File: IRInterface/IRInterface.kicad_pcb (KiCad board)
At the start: 2 copper layers, 27 x 33.5 mm, 25 parts, among them IC1 THVD1424RGTR, J2 RJHSE5E80, J3 FTSH-105-01-L-DV-007-K, Q1 SFH309, Q2 BC817, Q3 BC807, U1 74LVC1G17, U2 74LVC1G17, U3 STM32G030F6Px

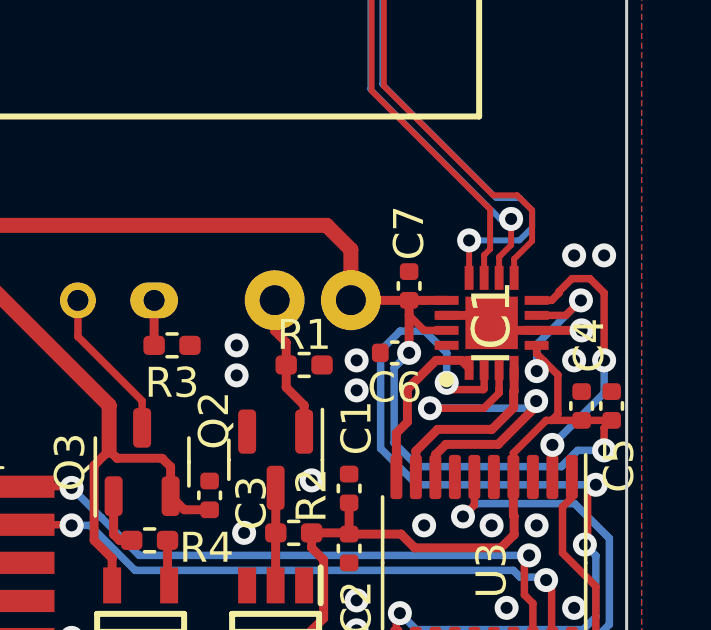
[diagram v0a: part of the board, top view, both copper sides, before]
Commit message: Fix review findings
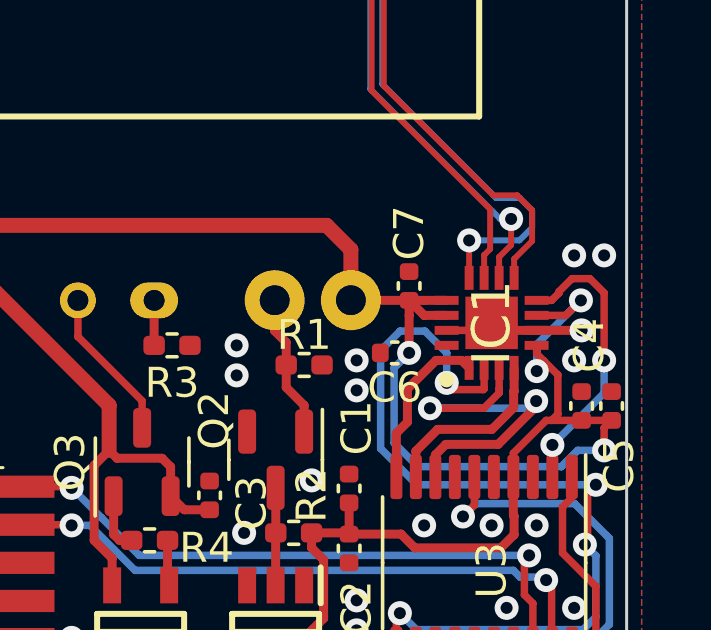
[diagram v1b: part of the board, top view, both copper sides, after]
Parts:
- R3: value 180R -> 150R
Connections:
- IC1 pad 14: GND -> VTref
- IC1 pad 15: VTref -> GND
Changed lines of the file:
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@@
         (effects (font (size 1 1) (thickness 0.15)))
     )
-    (fp_text value "180R" (at 0 1.17) (layer "F.Fab")
+    (fp_text value "150R" (at 0 1.17) (layer "F.Fab")
         (effects (font (size 1 1) (thickness 0.15)))
     )
@@
       (net 9 "DI+") (pinfunction "6") (pintype "passive"))
     (pad "7" thru_hole circle (at -6.09 0 180) (size 1.446 1.446) (drill 0.89) (layers "*.Cu" "*.Mask")
-      (net 15 "unconnected-(J2-Pad7)") (pinfunction "7") (pintype "passive"))
+      (net 15 "unconnected-(J2-Pad7)") (pinfunction "7") (pintype "passive+no_connect"))
     (pad "8" thru_hole circle (at -7.11 -1.78 180) (size 1.446 1.446) (drill 0.89) (layers "*.Cu" "*.Mask")
-      (net 16 "unconnected-(J2-Pad8)") (pinfunction "8") (pintype "passive"))
+      (net 16 "unconnected-(J2-Pad8)") (pinfunction "8") (pintype "passive+no_connect"))
     (pad "MH1" thru_hole circle (at 4.575 -0.89 180) (size 2.355 2.355) (drill 1.57) (layers "*.Cu" "*.Mask")
       (net 2 "GND") (pinfunction "MH1") (pintype "passive"))
@@
       (net 34 "VTref") (pinfunction "VIO") (pintype "passive"))
     (pad "14" smd rect (at 0.25 -1.5 90) (size 0.3 0.8) (layers "F.Cu" "F.Paste" "F.Mask")
-      (net 2 "GND") (pinfunction "VCC") (pintype "passive"))
+      (net 34 "VTref") (pinfunction "VCC") (pintype "passive"))
     (pad "15" smd rect (at -0.25 -1.5 90) (size 0.3 0.8) (layers "F.Cu" "F.Paste" "F.Mask")
-      (net 34 "VTref") (pinfunction "H/~{F}") (pintype "passive"))
+      (net 2 "GND") (pinfunction "H/~{F}") (pintype "passive"))
     (pad "16" smd rect (at -0.75 -1.5 90) (size 0.3 0.8) (layers "F.Cu" "F.Paste" "F.Mask")
       (net 13 "unconnected-(IC1-NC-Pad16)") (pinfunction "NC") (pintype "no_connect"))
@@
   (segment (start 17.25 12.96) (end 17.21 13) (width 0.5) (layer "F.Cu") (net 1))
   (segment (start 39 29.5) (end 40.5 29.5) (width 0.3) (layer "F.Cu") (net 2))
-  (segment (start 35.75 29) (end 36 29) (width 0.3) (layer "F.Cu") (net 2))
-  (segment (start 36 29) (end 37.25 29) (width 0.3) (layer "F.Cu") (net 2))
   (segment (start 37.25 29) (end 37.5 29.25) (width 0.3) (layer "F.Cu") (net 2))
+  (segment (start 37.25 29.5) (end 37.5 29.25) (width 0.25) (layer "F.Cu") (net 2))
   (segment (start 39 29.5) (end 37.75 29.5) (width 0.3) (layer "F.Cu") (net 2))
   (segment (start 37.75 29.5) (end 37.5 29.25) (width 0.3) (layer "F.Cu") (net 2))
+  (segment (start 36 29.5) (end 37.25 29.5) (width 0.25) (layer "F.Cu") (net 2))
   (via (at 31.5 34.5) (size 0.8) (drill 0.4) (layers "F.Cu" "B.Cu") (free) (net 2))
   (via (at 41.25 27) (size 0.8) (drill 0.4) (layers "F.Cu" "B.Cu") (free) (net 2))
@@
   (segment (start 34.990584 39.475) (end 40.550305 39.475) (width 0.25) (layer "B.Cu") (net 26))
   (segment (start 35.01035 34.646746) (end 33.8 33.436396) (width 0.25) (layer "B.Cu") (net 26))
-  (segment (start 35.25 29.5) (end 34.75 29) (width 0.25) (layer "F.Cu") (net 34))
   (segment (start 25.0125 33.7625) (end 24.75 33.5) (width 0.3) (layer "F.Cu") (net 34))
   (segment (start 39.317491 32.5) (end 38.225 33.592491) (width 0.25) (layer "F.Cu") (net 34))
@@
   (segment (start 31.5 36.25) (end 32.71 36.25) (width 0.3) (layer "F.Cu") (net 34))
   (segment (start 32 26) (end 18.75 26) (width 0.5) (layer "F.Cu") (net 34))
+  (segment (start 36 29) (end 35.25 29) (width 0.3) (layer "F.Cu") (net 34))
   (segment (start 34.939339 36.75) (end 37.810661 36.75) (width 0.3) (layer "F.Cu") (net 34))
   (segment (start 38.225 35.664339) (end 38.225 34.3875) (width 0.3) (layer "F.Cu") (net 34))
@@
   (segment (start 35.25 28.5) (end 32.814719 28.5) (width 0.3) (layer "F.Cu") (net 34))
   (segment (start 32.75 36.29) (end 34.479339 36.29) (width 0.3) (layer "F.Cu") (net 34))
-  (segment (start 36 29.5) (end 35.25 29.5) (width 0.25) (layer "F.Cu") (net 34))
   (segment (start 31.5 36.25) (end 31.5 36.75) (width 0.3) (layer "F.Cu") (net 34))
   (segment (start 37.810661 36.75) (end 38.25 36.310661) (width 0.3) (layer "F.Cu") (net 34))
@@
   (segment (start 32.814719 28.5) (end 32.808999 28.49428) (width 0.3) (layer "F.Cu") (net 34))
   (segment (start 26.5125 33.7625) (end 25.0125 33.7625) (width 0.3) (layer "F.Cu") (net 34))
+  (segment (start 35.25 29) (end 34.75 28.5) (width 0.3) (layer "F.Cu") (net 34))
   (segment (start 34.75 30.25) (end 34.75 29) (width 0.3) (layer "F.Cu") (net 34))
   (segment (start 41.25 32.75) (end 41.25 33.5) (width 0.25) (layer "F.Cu") (net 34))
